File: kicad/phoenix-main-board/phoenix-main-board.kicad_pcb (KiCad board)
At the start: 4 copper layers, 101.5 x 58 mm, 101 parts, among them U1 LM7705, U2 LT3092xDD, U3 TPS61222DCK, U4 Adafruit_Feather_nrf52840_Exp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, U5 TS5A3359, U6 TPS7A2033DQN, U7 OPA2380, U8 AD5242, U9 MCP3564

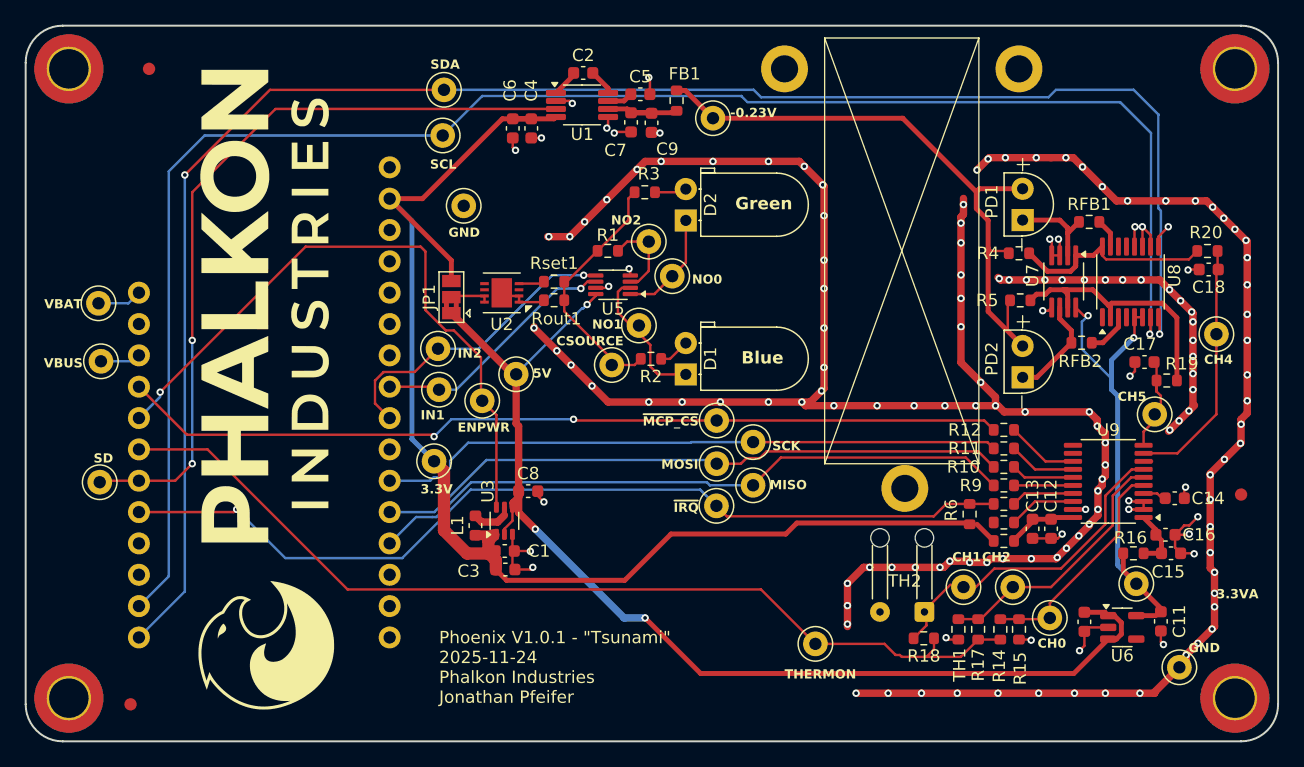
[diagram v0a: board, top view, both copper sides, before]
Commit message: PCB: Complete V1.1.0-Tornado
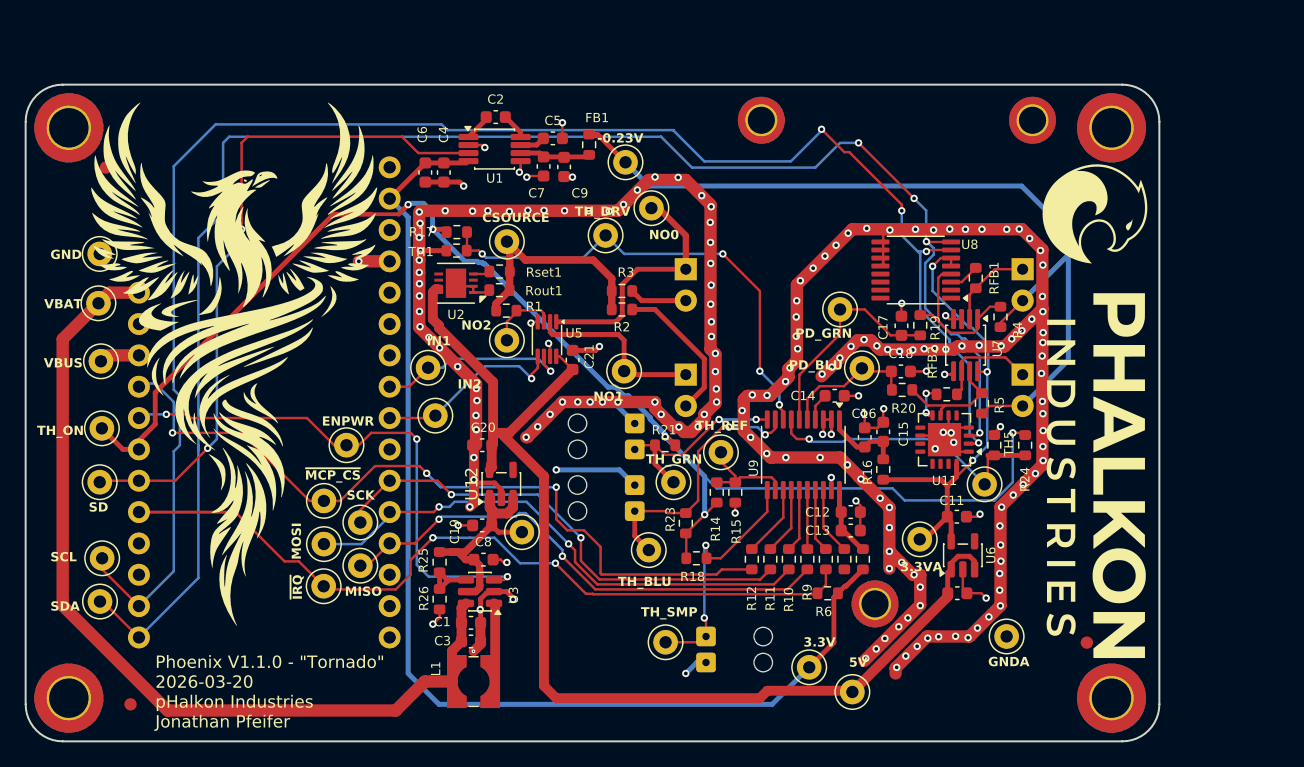
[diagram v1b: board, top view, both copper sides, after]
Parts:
- removed the G*** at (49.5, 49.5)
- removed the G*** at (97.0, 49.0)
- removed JP1: SolderJumper_3_Bridged12, Jumper:SolderJumper-3_P1.3mm_Bridged2Bar12_Pad1.0x1.5mm
- removed the REF** at (101.2, 57.5)
- removed the REF** at (110.5, 23.5)
- removed the REF** at (91.5, 23.5)
- added C19: 1uF, Capacitor_SMD:C_0603_1608Metric, F.Cu at (67.0, 60.5)
- added C20: 1uF, Capacitor_SMD:C_0603_1608Metric, F.Cu at (67.0, 54.0)
- added C21: 100nF, Capacitor_SMD:C_0603_1608Metric, F.Cu at (74.3, 47.1)
- added G***: LOGO, LOGO, F.Cu at (47.0, 47.5)
- added G***: LOGO, LOGO, F.Cu at (116.7, 51.2)
- added R21: 10k, Resistor_SMD:R_0603_1608Metric, F.Cu at (81.8, 54.0)
- added R23: 10k, Resistor_SMD:R_0603_1608Metric, F.Cu at (83.5, 60.3)
- added R24: 10k, Resistor_SMD:R_0603_1608Metric, F.Cu at (111.0, 54.0)
- added R25: 1M, Resistor_SMD:R_0603_1608Metric, F.Cu at (63.5, 63.5)
- added R26: 301k, Resistor_SMD:R_0603_1608Metric, F.Cu at (63.5, 66.5)
- added REF**: MountingHole_2.2mm_M2_DIN965_Pad_TopBottom, MountingHole:MountingHole_2.2mm_M2_DIN965_Pad_TopBottom, F.Cu at (98.8, 66.9)
- added REF**: MountingHole_2.2mm_M2_DIN965_Pad_TopBottom, MountingHole:MountingHole_2.2mm_M2_DIN965_Pad_TopBottom, F.Cu at (89.6, 27.7)
- added REF**: MountingHole_2.2mm_M2_DIN965_Pad_TopBottom, MountingHole:MountingHole_2.2mm_M2_DIN965_Pad_TopBottom, F.Cu at (111.6, 27.7)
- added TH3: GreenLEDThermistor, -ProjectLibrary:ThermistorWire, B.Cu at (79.4, 55.8)
- added TH4: BlueLED Thermistor, -ProjectLibrary:ThermistorWire, B.Cu at (79.4, 60.8)
- added TH5: GainStageThermistor, Resistor_SMD:R_0603_1608Metric, F.Cu at (108.5, 54.0)
- added TP31: TestPoint_Small, TestPoint:TestPoint_Keystone_5000-5004_Miniature, F.Cu at (97.0, 74.0)
- added TP32: TestPoint_Small, TestPoint:TestPoint_Keystone_5000-5004_Miniature, F.Cu at (77.0, 37.0)
- added TP33: TestPoint_Small, TestPoint:TestPoint_Keystone_5000-5004_Miniature, F.Cu at (81.9, 70.0)
- added TP34: TestPoint_Small, TestPoint:TestPoint_Keystone_5000-5004_Miniature, F.Cu at (86.3, 54.6)
- added U11: MCP41U83T, Package_DFN_QFN:Texas_RSA_VQFN-16-1EP_4x4mm_P0.65mm_EP2.7x2.7mm, F.Cu at (104.5, 53.6)
- added U12: TPS7A2050, Package_TO_SOT_SMD:SOT-23-5, F.Cu at (68.5, 57.1)
- D1, D2: moved to B.Cu
- L1: footprint Inductor_SMD:L_0603_1608Metric -> Inductor_SMD:L_Wuerth_WE-TPC-3816
- PD_Blue1: renamed from PD2; moved to B.Cu
- PD_Green1: renamed from PD1; moved to B.Cu
- R2: value 5 -> 0
- TH1: value EnclosureThermistor -> DriveStageThermistor
- TH2: footprint Connector_Wire:SolderWire-0.1sqmm_1x02_P3.6mm_D0.4mm_OD1mm_Relief -> -ProjectLibrary:ThermistorWire; moved to B.Cu
- U3: value TPS61222DCK -> MCP1640Bx-xCHY; footprint Package_TO_SOT_SMD:Texas_R-PDSO-G6 -> Package_TO_SOT_SMD:SOT-23-6
- U6: value TPS7A2033DQN -> TPS7A2033
- moved TP20 60.4 mm to (36.2, 52.6)
- moved R17 53.1 mm to (64.9, 36.7), turned to 0 degrees
- moved TH1 51.0 mm to (64.9, 38.2), turned to 180 degrees
- moved TP17 50.0 mm to (36.0, 66.7)
- moved TP27 49.2 mm to (80.5, 62.5)
- moved TP16 44.0 mm to (36.2, 63.2)
- moved TP28 39.4 mm to (82.5, 57.0)
- moved TP1 34.7 mm to (93.5, 72.0)
- moved TP18 32.5 mm to (54.2, 65.4)
- moved TP19 32.5 mm to (54.2, 58.5)
- moved TP3 32.5 mm to (57.1, 60.3)
- moved TP4 32.5 mm to (54.2, 62.0)
- moved TP5 32.5 mm to (57.1, 63.8)
- moved TP2 29.8 mm to (36.0, 38.5)
- moved C14 28.8 mm to (95.6, 50.0)
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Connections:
- C1 pad 1: +3.3V -> /VBAT
- C17 pad 1: /CH5 -> Net-(U9-CH1)
- C18 pad 1: /CH4 -> Net-(U9-CH0)
- C3 pad 1: +3.3V -> /VBAT
- C8 pad 1: +5V -> /5.2V BOOST
- L1 pad 1: +3.3V -> /VBAT
- L1 pad 2: Net-(U3-L) -> Net-(U3-SW)
- R14 pad 2: /CH0 -> /TH_REF
- R15 pad 1: /CH0 -> /TH_REF
- R17 pad 2: /CH1 -> /TH_DRV
- R18 pad 2: /CH2 -> /TH_SMP
- R19 pad 1: /CH5 -> Net-(U9-CH1)
- R19 pad 2: /PD2_SIG -> /PD_Green_SIG
- R20 pad 1: /CH4 -> Net-(U9-CH0)
- R20 pad 2: /PD1_SIG -> /PD_Blue_SIG
- R4 pad 1: /PD1_SIG -> /PD_Green_SIG
- R5 pad 1: /PD2_SIG -> /PD_Blue_SIG
- RFB1 pad 2: Net-(U8-W2) -> Net-(U8-W1)
- RFB2 pad 2: Net-(U8-W1) -> Net-(U11-P0W)
- TH1 pad 1: /CH1 -> /TH_DRV
- TH2 pad 1: /CH2 -> /TH_SMP
- TP12 pad 1: +5V -> /5.2V BOOST
- TP13 pad 1: Net-(U4-VBAT) -> /VBAT
- TP24 pad 1: /CH0 -> Net-(U9-CH0)
- TP25 pad 1: /CH1 -> Net-(U9-CH1)
- TP26 pad 1: /CH2 -> /TH_GAIN
- TP27 pad 1: /CH4 -> /TH_BLU
- TP28 pad 1: /CH5 -> /TH_GRN
- U2 pad 7: Net-(JP1-C) -> +5V
- U2 pad 8: Net-(JP1-C) -> +5V
- U3 pad 1: +3.3V -> Net-(U3-SW)
- U3 pad 2: +5V -> GND
- U3 pad 3: GND -> /EnablePower
- U3 pad 4: +5V -> Net-(U3-V_{FB})
- U3 pad 5: Net-(U3-L) -> /5.2V BOOST
- U3 pad 6: /EnablePower -> /VBAT
- U4 pad 17: Net-(U4-VBAT) -> /VBAT
- U7 pad 1: /PD1_SIG -> /PD_Green_SIG
- U7 pad 7: /PD2_SIG -> /PD_Blue_SIG
- U8 pad 15: Net-(U8-W2) -> unconnected-(U8-W2-Pad15)
- U8 pad 16: /PD1_SIG -> unconnected-(U8-A2-Pad16)
- U8 pad 2: /PD2_SIG -> unconnected-(U8-A1-Pad2)
- U8 pad 4: unconnected-(U8-B1-Pad4) -> /PD_Green_SIG
- U9 pad 10: /CH5 -> /TH_GRN
- U9 pad 11: /CH6 -> /TH_SMP
- U9 pad 12: /CH7 -> /TH_REF
- U9 pad 5: /CH0 -> Net-(U9-CH0)
- U9 pad 6: /CH1 -> Net-(U9-CH1)
- U9 pad 7: /CH2 -> /TH_GAIN
- U9 pad 8: /CH3 -> /TH_DRV
- U9 pad 9: /CH4 -> /TH_BLU
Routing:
- net /VBAT: track 0.00 -> 72.3 mm
- net /TH_DRV: track 0.00 -> 39.4 mm, vias 0 -> 4
- net /Thermistor_On: track 79.1 -> 112.4 mm, vias 0 -> 5
- net /CH2: track 25.5 -> 0.00 mm
- net /TH_GAIN: track 0.00 -> 24.2 mm, vias 0 -> 1
- net /TH_BLU: track 0.00 -> 21.9 mm, vias 0 -> 2
- net /CH1: track 21.2 -> 0.00 mm
- net /PD2_SIG: track 21.0 -> 0.00 mm
- net /CH4: track 20.4 -> 0.00 mm
- net /TH_SMP: track 0.00 -> 20.3 mm, vias 0 -> 2
- net /5.2V BOOST: track 0.00 -> 19.7 mm
- net /CH0: track 18.5 -> 0.00 mm
- net Net-(U9-CH1): track 0.00 -> 17.7 mm
- net -0.23V: track 51.9 -> 69.4 mm
- net /PD1_SIG: track 17.0 -> 0.00 mm
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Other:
- board size 101.5 x 58 mm -> 91.9 x 53.2 mm
- board text added: "GNDA"
- board text added: "PD_BLU"
- board text added: "PD_GRN"
- board text added: "Phoenix V1.1.0 - {dblquote}Tornado{dblquote} 2026-03-20 pHalkon Industries Jonathan Pfeifer"
- board text added: "TH_BLU"
- board text added: "TH_DRV"
- board text added: "TH_GRN"
- board text added: "TH_ON"
- board text added: "TH_REF"
- board text added: "TH_SMP"
- board text removed: "CH0"
- board text removed: "CH1"
- board text removed: "CH2"
- board text removed: "CH4"
- board text removed: "CH5"
- board text removed: "Phoenix V1.0.1 - {dblquote}Tsunami{dblquote} 2025-11-24 Phalkon Industries Jonathan Pfeifer"
- board text removed: "THERMON"
